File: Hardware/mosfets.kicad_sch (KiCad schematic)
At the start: 15 parts, among them Q1 IRFS7530, Q2 IRFS7530, Q3 IRFS7530, Q4 IRFS7530, Q5 IRFS7530, Q6 IRFS7530

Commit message: chatting to fang
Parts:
- R28, R29, R30, R34, R35, R36, R42, R43, R46: footprint CRF1:SMD-0603_r -> Resistor_SMD:R_0603_1608Metric
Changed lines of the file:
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@@
 			)
 		)
-		(property "Footprint" "CRF1:SMD-0603_r"
+		(property "Footprint" "Resistor_SMD:R_0603_1608Metric"
 			(at 199.39 102.87 0)
 			(effects
@@
 			)
 		)
-		(property "Footprint" "CRF1:SMD-0603_r"
+		(property "Footprint" "Resistor_SMD:R_0603_1608Metric"
 			(at 119.38 102.87 0)
 			(effects
@@
 			)
 		)
-		(property "Footprint" "CRF1:SMD-0603_r"
+		(property "Footprint" "Resistor_SMD:R_0603_1608Metric"
 			(at 111.76 95.25 0)
 			(effects
@@
 			)
 		)
-		(property "Footprint" "CRF1:SMD-0603_r"
+		(property "Footprint" "Resistor_SMD:R_0603_1608Metric"
 			(at 111.76 71.12 0)
 			(effects
@@
 			)
 		)
-		(property "Footprint" "CRF1:SMD-0603_r"
+		(property "Footprint" "Resistor_SMD:R_0603_1608Metric"
 			(at 151.13 71.12 0)
 			(effects
@@
 			)
 		)
-		(property "Footprint" "CRF1:SMD-0603_r"
+		(property "Footprint" "Resistor_SMD:R_0603_1608Metric"
 			(at 151.13 95.25 0)
 			(effects
@@
 			)
 		)
-		(property "Footprint" "CRF1:SMD-0603_r"
+		(property "Footprint" "Resistor_SMD:R_0603_1608Metric"
 			(at 191.77 95.25 0)
 			(effects
@@
 			)
 		)
-		(property "Footprint" "CRF1:SMD-0603_r"
+		(property "Footprint" "Resistor_SMD:R_0603_1608Metric"
 			(at 191.77 71.12 0)
 			(effects
@@
 			)
 		)
-		(property "Footprint" "CRF1:SMD-0603_r"
+		(property "Footprint" "Resistor_SMD:R_0603_1608Metric"
 			(at 151.13 102.87 0)
 			(effects

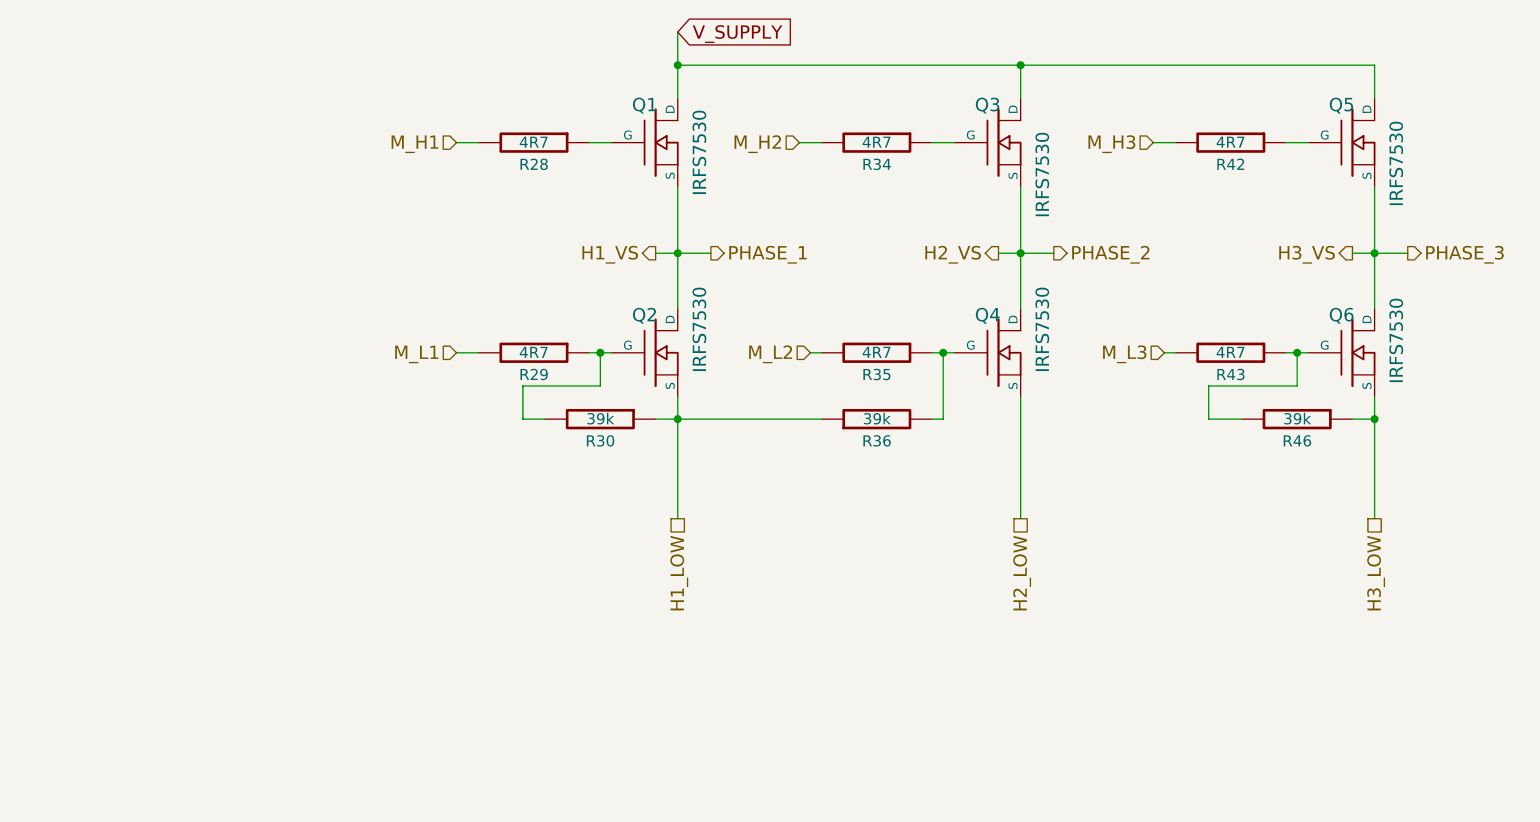
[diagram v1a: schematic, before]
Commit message: close to 1st done
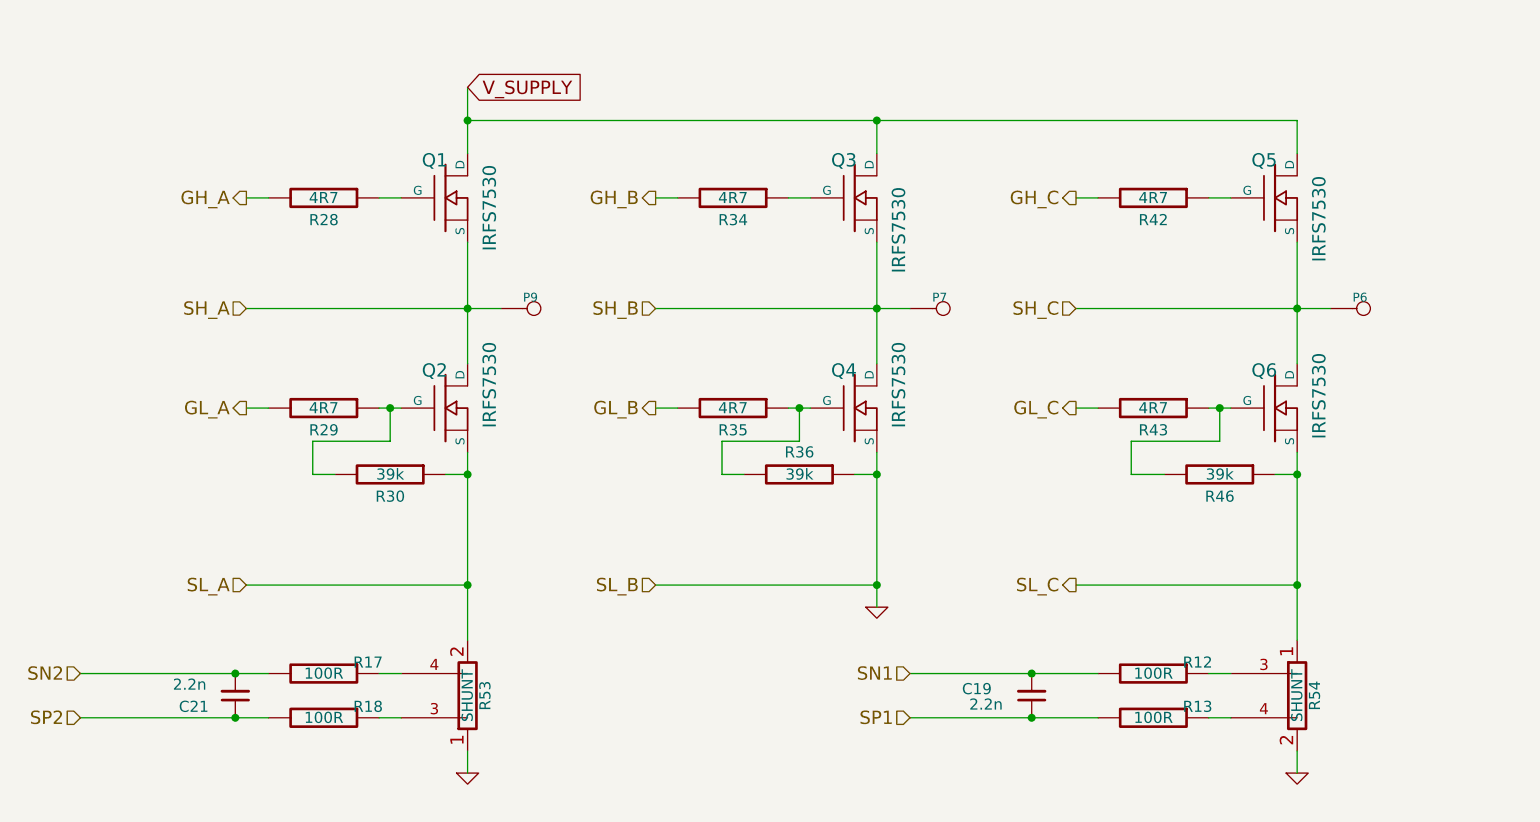
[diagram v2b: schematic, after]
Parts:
- added C19, C21: 2.2n, Capacitor_SMD:C_0603_1608Metric, symbol Device:C_Small
- added P6: MOTOR1, CRF1:1PAD_4x5mm, symbol BLDC_4-rescue:CONN_1
- added P7: MOTOR2, CRF1:1PAD_4x5mm, symbol BLDC_4-rescue:CONN_1
- added P9: MOTOR3, CRF1:1PAD_4x5mm, symbol BLDC_4-rescue:CONN_1
- added R12, R13, R17, R18: 100R, Resistor_SMD:R_0603_1608Metric, symbol BLDC_4-rescue:R-RESCUE-BLDC_4
- added R53, R54: SHUNT, CRF1:WSLP2726, symbol crf_1:SHUNT
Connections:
- net H1_LOW renamed SL_A
- net SL_A: now also R53.2; no longer R36.1
- net H1_VS renamed SH_A
- net SH_A: now also P9.1
- net H2_LOW renamed GND
- net GND: now also R36.1, R53.1, R54.2
- net H2_VS renamed SH_B
- net SH_B: now also P7.1
- net H3_LOW renamed SL_C
- net SL_C: now also R54.1
- net H3_VS renamed SH_C
- net SH_C: now also P6.1
- net M_H1 renamed GH_A
- net M_H2 renamed GH_B
- net M_H3 renamed GH_C
- net M_L1 renamed GL_A
- net M_L2 renamed GL_B
- net M_L3 renamed GL_C
- new net: R18.1, R53.3
- new net: R17.1, R53.4
- new net: R12.1, R54.3
- new net: R13.1, R54.4
- new net SN1: C19.2, R12.2
- new net SN2: C21.2, R17.2
- new net SP1: C19.1, R13.2
- new net SP2: C21.1, R18.2
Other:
- moved on the sheet: Q1, Q2, Q3, Q4, Q5, Q6, R28, R29, R30, R34, R35, R36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

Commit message: changes made post will's review
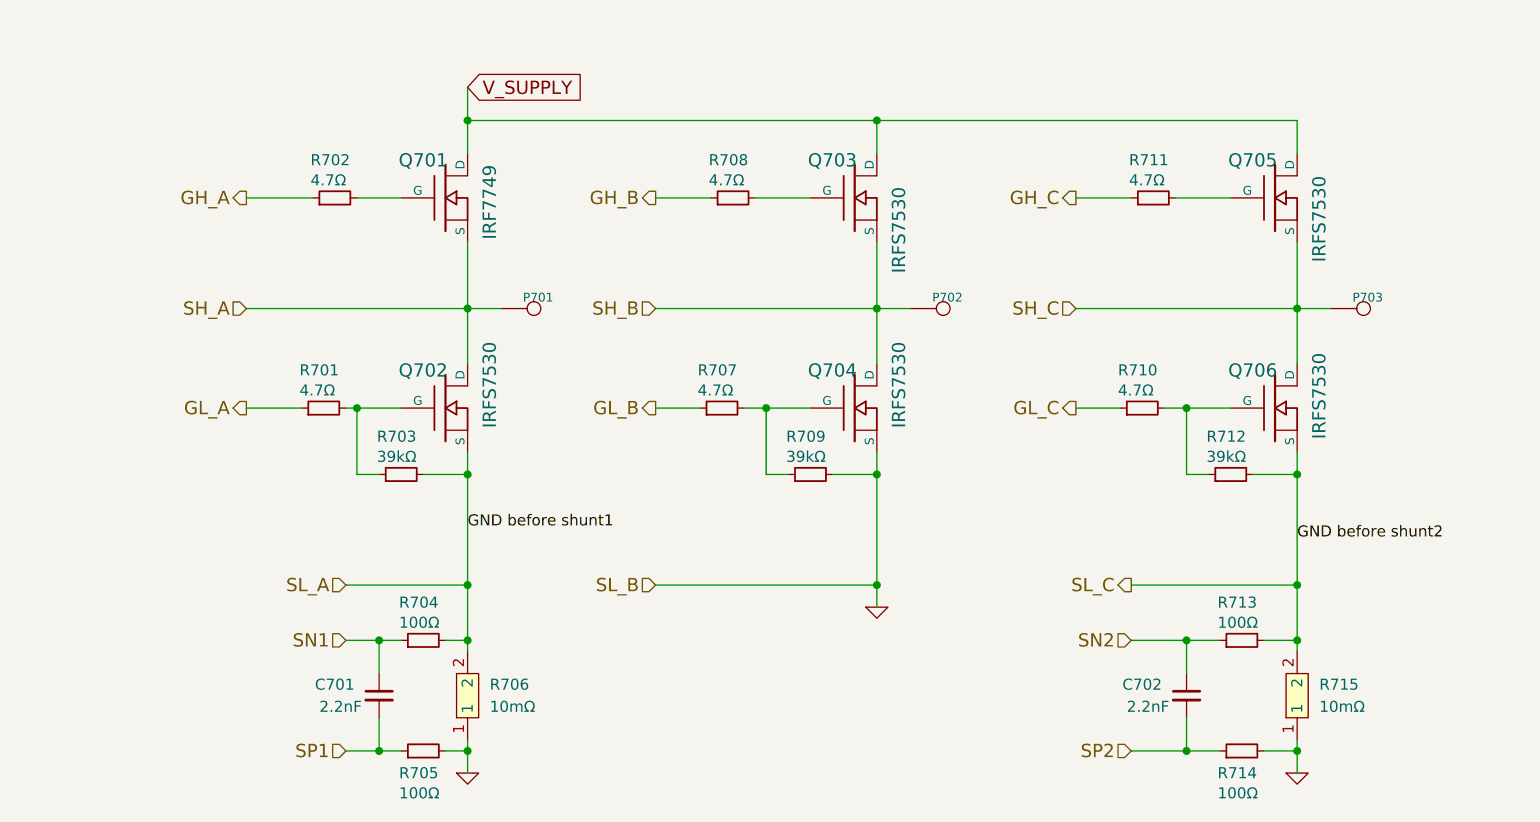
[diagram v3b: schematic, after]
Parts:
- removed C19, C21: 2.2n, Capacitor_SMD:C_0603_1608Metric, symbol Device:C_Small
- removed R12, R13, R17, R18: 100R, Resistor_SMD:R_0603_1608Metric, symbol BLDC_4-rescue:R-RESCUE-BLDC_4
- removed R28, R29, R34, R35, R42, R43: 4R7, Resistor_SMD:R_0603_1608Metric, symbol BLDC_4-rescue:R-RESCUE-BLDC_4
- removed R30, R36, R46: 39k, Resistor_SMD:R_0603_1608Metric, symbol BLDC_4-rescue:R-RESCUE-BLDC_4
- removed R53, R54: SHUNT, CRF1:WSLP2726, symbol crf_1:SHUNT
- added C701, C702: 2.2nF, Capacitor_SMD:C_0402_1005Metric, symbol Device:C_Small
- added R701, R702, R707, R708, R710, R711: 4.7Ω, Resistor_SMD:R_0603_1608Metric, symbol Device:R_Small
- added R703, R709, R712: 39kΩ, Resistor_SMD:R_0402_1005Metric, symbol Device:R_Small
- added R704, R705, R713, R714: 100Ω, Resistor_SMD:R_0402_1005Metric, symbol Device:R_Small
- added R706, R715: 10mΩ, easyeda2kicad:RES-SMD_L7.1-W4.6_HOXLR2818, symbol easyeda2kicad:HORCG28185R010F4T
- Q701: renamed from Q1; value IRFS7530 -> IRF7749
- renumbered P9 to P701, P7 to P702, P6 to P703, Q2 to Q702, Q3 to Q703, Q4 to Q704, Q5 to Q705, Q6 to Q706
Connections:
- net GH_A: now also R702.1
- net GH_B: now also R708.1
- net GH_C: now also R711.1
- net GL_A: now also R701.1
- net GL_B: now also R707.1
- net GL_C: now also R710.1
- net GND: now also R705.2, R706.1, R709.2, R714.2, R715.1
- net SL_A: now also R703.2, R704.2, R706.2
- net SL_C: now also R712.2, R713.2, R715.2
- net SN1: now also C701.1, R704.1
- net SN2: now also C702.1, R713.1
- net SP1: now also C701.2, R705.1
- net SP2: now also C702.2, R714.1
- net at Q706.G: now also R710.2, R712.1
- net at Q702.G: now also R701.2, R703.1
- net at Q701.G: now also R702.2
- net at Q703.G: now also R708.2
- net at Q704.G: now also R707.2, R709.1
- net at Q705.G: now also R711.2
